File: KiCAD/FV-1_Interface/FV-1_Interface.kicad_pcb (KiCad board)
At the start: 2 copper layers, 29 parts, among them J1 ERK_PWR, J2 TP_GND, J4 IN, J5 OUT, J6 FX_OUT, J7 FX_IN, U2 TL072

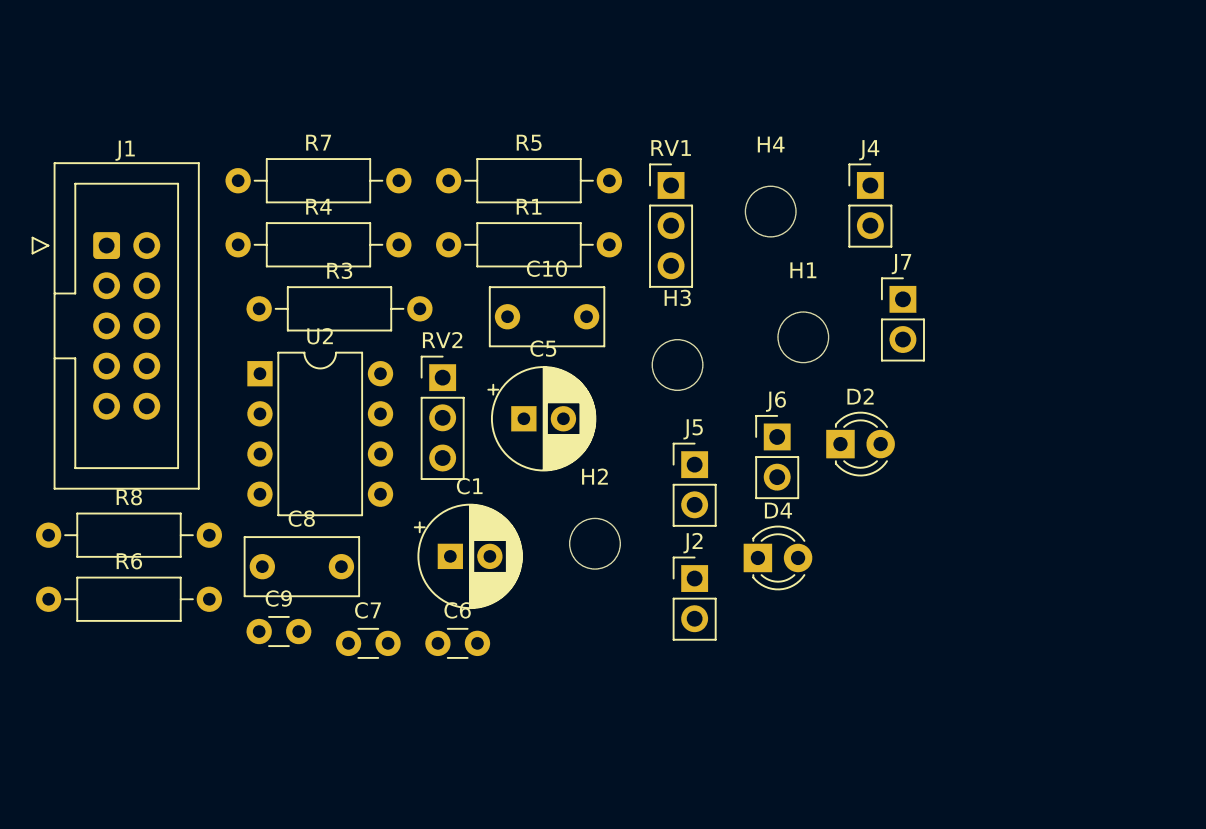
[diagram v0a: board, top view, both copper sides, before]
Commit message: FV-1 Interface module
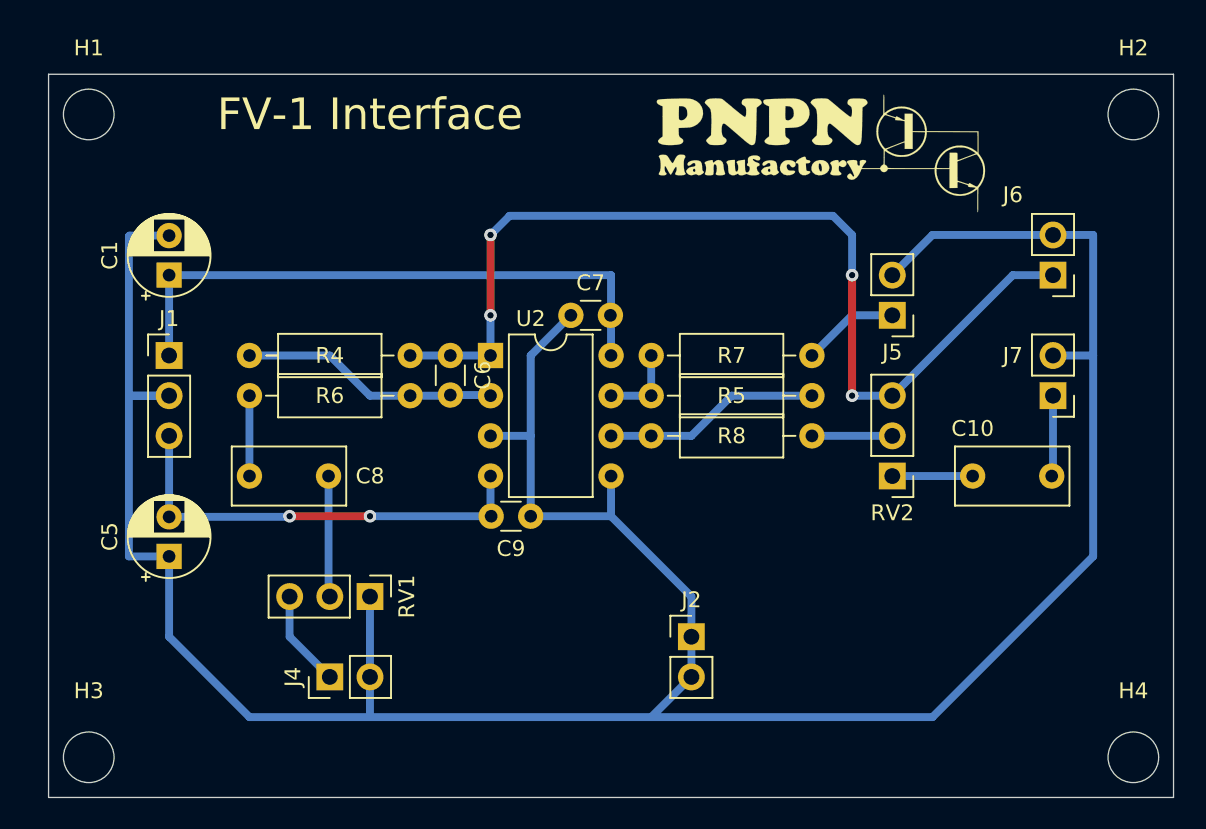
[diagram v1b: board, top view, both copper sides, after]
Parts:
- removed D2: RED, LED_THT:LED_D3.0mm
- removed D4: BLUE, LED_THT:LED_D3.0mm
- removed R1, R3: 3.3k, Resistor_THT:R_Axial_DIN0207_L6.3mm_D2.5mm_P10.16mm_Horizontal
- added G***: LOGO, myfootprint:Silk_PNPN_Thyristor_1200dpi, F.Cu at (174.6, 81.3)
- added G***: LOGO, myfootprint:Silk_PNPN_Manufactory_600dpi, F.Cu at (164.5, 80.0)
- C1, C5: footprint Capacitor_THT:CP_Radial_D6.3mm_P2.50mm -> Capacitor_THT:CP_Radial_D5.0mm_P2.50mm
- J1: value ERK_PWR -> PWR; footprint Connector_IDC:IDC-Header_2x05_P2.54mm_Vertical -> Connector_PinHeader_2.54mm:PinHeader_1x03_P2.54mm_Vertical
- moved H1 47.3 mm to (121.9, 78.7)
- moved J4 46.2 mm to (137.2, 114.3), turned to 90 degrees
- moved H3 44.7 mm to (121.9, 119.4)
- moved H2 43.5 mm to (188.0, 78.7)
- moved H4 41.4 mm to (188.0, 119.4)
- moved R8 38.6 mm to (157.5, 99.1)
- moved R7 37.9 mm to (167.6, 94.0), turned to 180 degrees
- moved RV1 32.2 mm to (139.7, 109.2), turned to 270 degrees
- moved C10 31.1 mm to (177.8, 101.6)
- moved RV2 29.1 mm to (172.7, 101.6), turned to 180 degrees
- moved R6 26.2 mm to (142.2, 96.5), turned to 180 degrees
- moved C1 25.1 mm to (127.0, 88.9), turned to 90 degrees
- moved C7 25.1 mm to (152.4, 91.4)
- moved C5 24.1 mm to (127.0, 106.7), turned to 90 degrees
- moved J6 20.2 mm to (182.9, 88.9), turned to 180 degrees
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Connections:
- C1 pad 2: Net-(C1-Pad2) -> GND
- C5 pad 1: Net-(C1-Pad2) -> GND
- J1 pad 1: -12V -> +12V
- J1 pad 2: (no net) -> GND
- J1 pad 3: (no net) -> -12V
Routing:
- net GND: track 0.00 -> 183.6 mm
- net Net-(C6-Pad1): track 0.00 -> 62.6 mm, vias 0 -> 4
- net +12V: track 0.00 -> 38.1 mm
- net -12V: track 0.00 -> 28.1 mm, vias 0 -> 2
- net Net-(C6-Pad2): track 0.00 -> 16.3 mm
- net Net-(R5-Pad2): track 0.00 -> 13.8 mm
- net Net-(C8-Pad2): track 0.00 -> 7.65 mm
- net Net-(J5-Pad1): track 0.00 -> 6.13 mm
- net Net-(J4-Pad1): track 0.00 -> 6.13 mm
- net Net-(C10-Pad2): track 0.00 -> 5.11 mm
- net Net-(R8-Pad2): track 0.00 -> 5.08 mm
- net Net-(C10-Pad1): track 0.00 -> 5.08 mm
- net Net-(C8-Pad1): track 0.00 -> 5.08 mm
- net Net-(R5-Pad1): track 0.00 -> 5.08 mm
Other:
- board outline added: 71.1 x 45.7 mm
- board text added: "FV-1 Interface"
